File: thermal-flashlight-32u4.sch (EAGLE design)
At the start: 30 parts, among them IC2 MCP73831, IC3 ATMEGA32U4-AU, IC4 MCP1700-33, J1 AYZ0202, J2 1X2-3.5MM, Q4 BSS123, U1 MLX90614_, X1 USBSMD, X3 8MHz

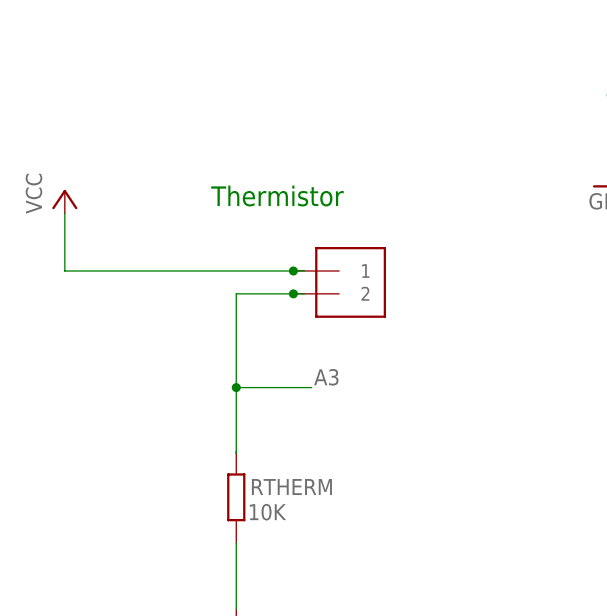
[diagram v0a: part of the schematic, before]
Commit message: update
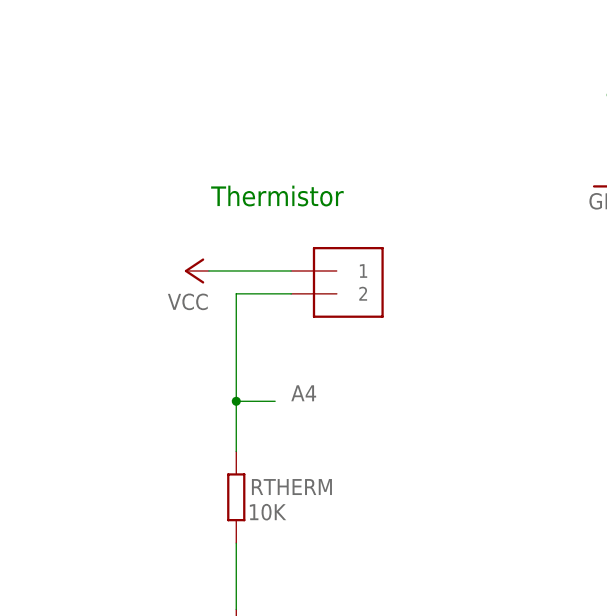
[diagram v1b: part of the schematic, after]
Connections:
- net A3: no longer J2.2, RTHERM.2
- net A4: now also J2.2, RTHERM.2
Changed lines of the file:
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@@
 <part name="GND1" library="SparkFun" deviceset="GND" device=""/>
 <part name="RTHERM" library="rcl" deviceset="R-EU_" device="R0805" value="10K"/>
-<part name="P+5" library="supply1" deviceset="VCC" device=""/>
 <part name="GND9" library="supply1" deviceset="GND" device=""/>
 <part name="GND10" library="supply1" deviceset="GND" device=""/>
@@
 <part name="P+1" library="supply1" deviceset="VCC" device=""/>
 <part name="SV1" library="con-lstb" deviceset="MA03-2" device=""/>
+<part name="P+7" library="supply1" deviceset="VCC" device=""/>
 </parts>
 <sheets>
@@
 <attribute name="VALUE" x="158.75" y="99.06" size="1.778" layer="96"/>
 </instance>
-<instance part="J2" gate="G$1" x="-30.734" y="-20.828"/>
+<instance part="J2" gate="G$1" x="-30.988" y="-20.828"/>
 <instance part="GND1" gate="1" x="-42.164" y="-58.42"/>
 <instance part="RTHERM" gate="G$1" x="-42.164" y="-43.434" smashed="yes" rot="R90">
@@
 <attribute name="VALUE" x="-40.894" y="-45.974" size="1.778" layer="96"/>
 </instance>
-<instance part="P+5" gate="VCC" x="-61.214" y="-9.398"/>
 <instance part="GND9" gate="1" x="19.812" y="-19.05"/>
 <instance part="GND10" gate="1" x="-0.508" y="-8.89"/>
@@
 <instance part="P+1" gate="VCC" x="143.51" y="53.086"/>
 <instance part="SV1" gate="1" x="127.762" y="-13.97"/>
+<instance part="P+7" gate="VCC" x="-47.752" y="-18.288" rot="R90"/>
 </instances>
 <busses>
@@
 </segment>
 <segment>
-<wire x1="-34.544" y1="-18.288" x2="-35.814" y2="-18.288" width="0.1524" layer="91"/>
-<pinref part="J2" gate="G$1" pin="1"/>
-<wire x1="-35.814" y1="-18.288" x2="-61.214" y2="-18.288" width="0.1524" layer="91"/>
-<junction x="-35.814" y="-18.288"/>
-<wire x1="-61.214" y1="-18.288" x2="-61.214" y2="-11.938" width="0.1524" layer="91"/>
-<pinref part="P+5" gate="VCC" pin="VCC"/>
-</segment>
-<segment>
 <wire x1="19.812" y1="41.91" x2="19.812" y2="44.45" width="0.1524" layer="91"/>
 <wire x1="7.112" y1="41.91" x2="19.812" y2="41.91" width="0.1524" layer="91"/>
@@
 <label x="138.176" y="-13.716" size="1.778" layer="95"/>
 </segment>
+<segment>
+<pinref part="J2" gate="G$1" pin="1"/>
+<pinref part="P+7" gate="VCC" pin="VCC"/>
+<wire x1="-45.212" y1="-18.288" x2="-36.068" y2="-18.288" width="0.1524" layer="91"/>
+</segment>
 </net>
 <net name="SCK" class="0">
@@
 </net>
 <net name="A3" class="0">
-<segment>
-<wire x1="-34.544" y1="-20.828" x2="-35.814" y2="-20.828" width="0.1524" layer="91"/>
-<wire x1="-35.814" y1="-20.828" x2="-42.164" y2="-20.828" width="0.1524" layer="91"/>
-<wire x1="-42.164" y1="-20.828" x2="-42.164" y2="-31.242" width="0.1524" layer="91"/>
-<pinref part="J2" gate="G$1" pin="2"/>
-<junction x="-35.814" y="-20.828"/>
-<pinref part="RTHERM" gate="G$1" pin="2"/>
-<wire x1="-42.164" y1="-31.242" x2="-42.164" y2="-38.354" width="0.1524" layer="91"/>
-<wire x1="-42.164" y1="-38.354" x2="-42.164" y2="-38.608" width="0.1524" layer="91"/>
-<wire x1="-42.164" y1="-31.242" x2="-33.782" y2="-31.242" width="0.1524" layer="91"/>
-<junction x="-42.164" y="-31.242"/>
-<label x="-33.528" y="-30.988" size="1.778" layer="95"/>
-</segment>
 <segment>
 <pinref part="IC3" gate="G$1" pin="PF4(ADC4/TCK)"/>
@@
 <label x="70.866" y="55.118" size="1.778" layer="95"/>
 </segment>
-</net>
+<segment>
+<pinref part="RTHERM" gate="G$1" pin="2"/>
+<wire x1="-42.164" y1="-38.354" x2="-42.164" y2="-32.766" width="0.1524" layer="91"/>
+<wire x1="-42.164" y1="-32.766" x2="-42.164" y2="-20.828" width="0.1524" layer="91"/>
+<wire x1="-42.164" y1="-20.828" x2="-36.068" y2="-20.828" width="0.1524" layer="91"/>
+<pinref part="J2" gate="G$1" pin="2"/>
+<wire x1="-42.164" y1="-32.766" x2="-37.846" y2="-32.766" width="0.1524" layer="91"/>
+<junction x="-42.164" y="-32.766"/>
+<label x="-36.068" y="-32.766" size="1.778" layer="95"/>
+</segment>
+</net>

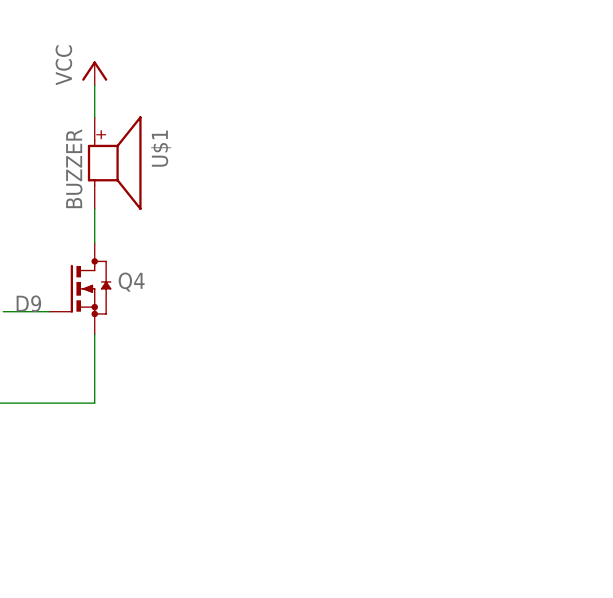
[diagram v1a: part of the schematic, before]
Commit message: update
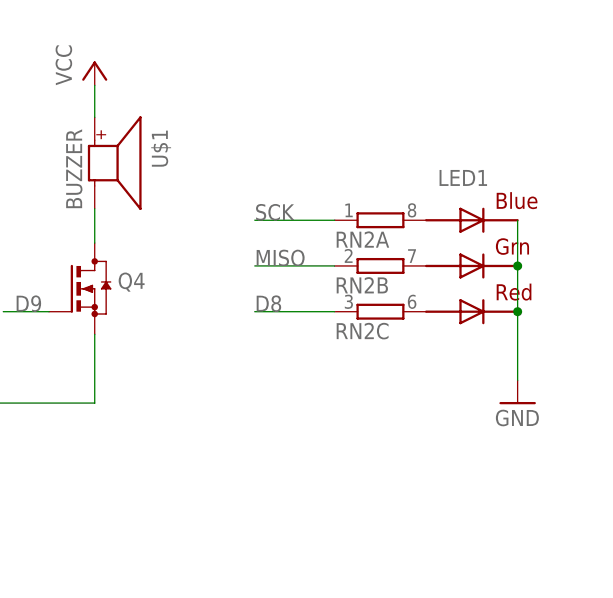
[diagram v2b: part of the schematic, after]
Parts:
- added LED1: RGBLED5050, adafruit:RGBLED5050
- added RN2: (no value), resistor-dil:4R-NEXB38V
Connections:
- new net N$12: LED1.RED_A, RN2C.2
- new net N$2: LED1.BLUE_A, RN2A.2
- new net N$3: LED1.GREEN_A, RN2B.2
- net D8: now also RN2C.1
- net GND: now also LED1.BLUE_C, LED1.GREEN_C, LED1.RED_C
- net MISO: now also RN2B.1
- net SCK: now also RN2A.1
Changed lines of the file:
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@@
 <setting verticaltext="up"/>
 </settings>
-<grid distance="0.01" unitdist="inch" unit="inch" style="lines" multiple="1" display="no" altdistance="0.01" altunitdist="inch" altunit="inch"/>
+<grid distance="0.1" unitdist="inch" unit="inch" style="lines" multiple="1" display="no" altdistance="0.01" altunitdist="inch" altunit="inch"/>
 <layers>
 <layer number="1" name="Top" color="4" fill="1" visible="no" active="no"/>
@@
 <part name="SV1" library="con-lstb" deviceset="MA03-2" device=""/>
 <part name="P+7" library="supply1" deviceset="VCC" device=""/>
+<part name="LED1" library="adafruit" deviceset="RGBLED" device="5050"/>
+<part name="RN2" library="resistor-dil" deviceset="4R-N" device="EXB38V"/>
+<part name="GND3" library="supply1" deviceset="GND" device=""/>
 </parts>
 <sheets>
@@
 <instance part="SV1" gate="1" x="127.762" y="-13.97"/>
 <instance part="P+7" gate="VCC" x="-47.752" y="-18.288" rot="R90"/>
+<instance part="LED1" gate="G$1" x="185.42" y="30.48"/>
+<instance part="RN2" gate="A" x="175.26" y="35.56"/>
+<instance part="RN2" gate="B" x="175.26" y="30.48"/>
+<instance part="RN2" gate="C" x="175.26" y="25.4"/>
+<instance part="GND3" gate="1" x="190.5" y="15.24"/>
 </instances>
 <busses>
@@
 <label x="137.922" y="-16.51" size="1.778" layer="95"/>
 </segment>
+<segment>
+<pinref part="LED1" gate="G$1" pin="BLUE_C"/>
+<pinref part="LED1" gate="G$1" pin="GREEN_C"/>
+<wire x1="190.5" y1="35.56" x2="190.5" y2="30.48" width="0.1524" layer="91"/>
+<pinref part="LED1" gate="G$1" pin="RED_C"/>
+<wire x1="190.5" y1="30.48" x2="190.5" y2="25.4" width="0.1524" layer="91"/>
+<junction x="190.5" y="30.48"/>
+<wire x1="190.5" y1="25.4" x2="190.5" y2="17.78" width="0.1524" layer="91"/>
+<junction x="190.5" y="25.4"/>
+<pinref part="GND3" gate="1" pin="GND"/>
+</segment>
 </net>
 <net name="VBUS" class="0">
@@
 <pinref part="IC3" gate="G$1" pin="PB1(SCK)"/>
 </segment>
+<segment>
+<wire x1="170.18" y1="35.56" x2="161.29" y2="35.56" width="0.1524" layer="91"/>
+<label x="161.29" y="35.56" size="1.778" layer="95"/>
+<pinref part="RN2" gate="A" pin="1"/>
+</segment>
 </net>
 <net name="MISO" class="0">
@@
 <label x="70.612" y="13.97" size="1.778" layer="95"/>
 <pinref part="IC3" gate="G$1" pin="PB3(PDO/MISO)"/>
+</segment>
+<segment>
+<wire x1="170.18" y1="30.48" x2="161.29" y2="30.48" width="0.1524" layer="91"/>
+<label x="161.29" y="30.48" size="1.778" layer="95"/>
+<pinref part="RN2" gate="B" pin="1"/>
 </segment>
 </net>
@@
 <wire x1="68.072" y1="16.51" x2="73.914" y2="16.51" width="0.1524" layer="91"/>
 <label x="74.168" y="16.764" size="1.778" layer="95"/>
+</segment>
+<segment>
+<wire x1="170.18" y1="25.4" x2="161.29" y2="25.4" width="0.1524" layer="91"/>
+<label x="161.29" y="25.4" size="1.778" layer="95"/>
+<pinref part="RN2" gate="C" pin="1"/>
 </segment>
 </net>
@@
 </segment>
 </net>
+<net name="N$2" class="0">
+<segment>
+<pinref part="LED1" gate="G$1" pin="BLUE_A"/>
+<pinref part="RN2" gate="A" pin="2"/>
+</segment>
+</net>
+<net name="N$3" class="0">
+<segment>
+<pinref part="LED1" gate="G$1" pin="GREEN_A"/>
+<pinref part="RN2" gate="B" pin="2"/>
+</segment>
+</net>
+<net name="N$12" class="0">
+<segment>
+<pinref part="LED1" gate="G$1" pin="RED_A"/>
+<pinref part="RN2" gate="C" pin="2"/>
+</segment>
+</net>
